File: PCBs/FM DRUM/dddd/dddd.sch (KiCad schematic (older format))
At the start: 44 parts, among them J1 Conn_02x12_Odd_Even, J2 Conn_01x03, J3 Conn_01x03, J4 Conn_01x03, J5 Conn_01x03, J6 Conn_01x03, J7 Conn_01x03, SW1 SW_DIP_x06, U1 LM555xM, U2 LM555xM, U3 MCP46x2, U4 LM555xM, U5 LM555xM, U6 MCP46x2, U7 MCP46x2, U8 TL072

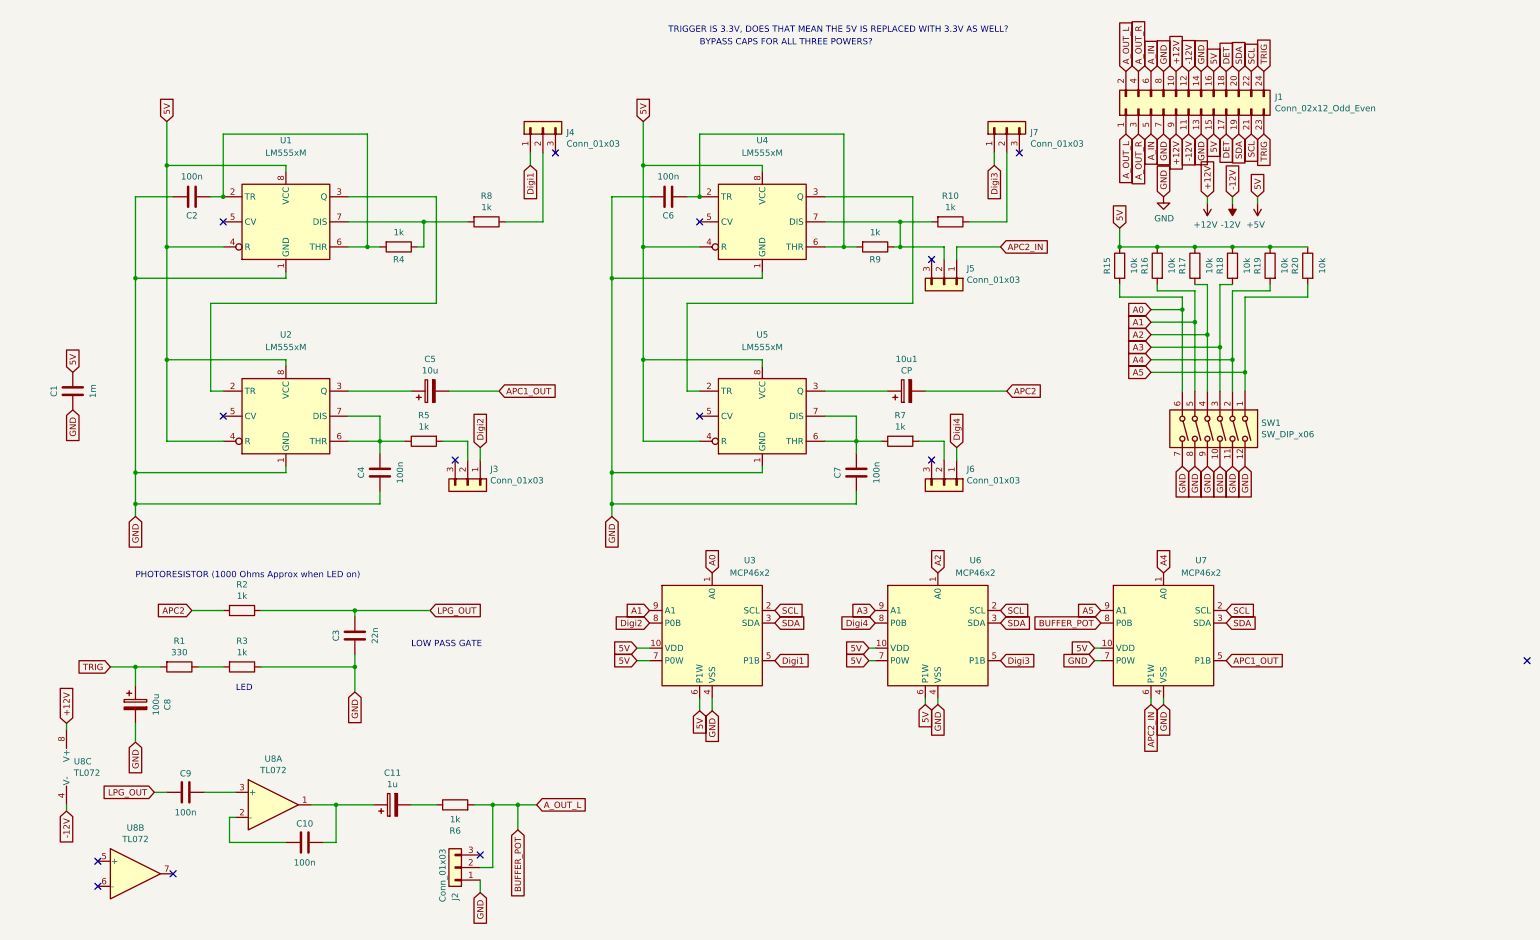
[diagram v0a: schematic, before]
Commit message: Add files via upload
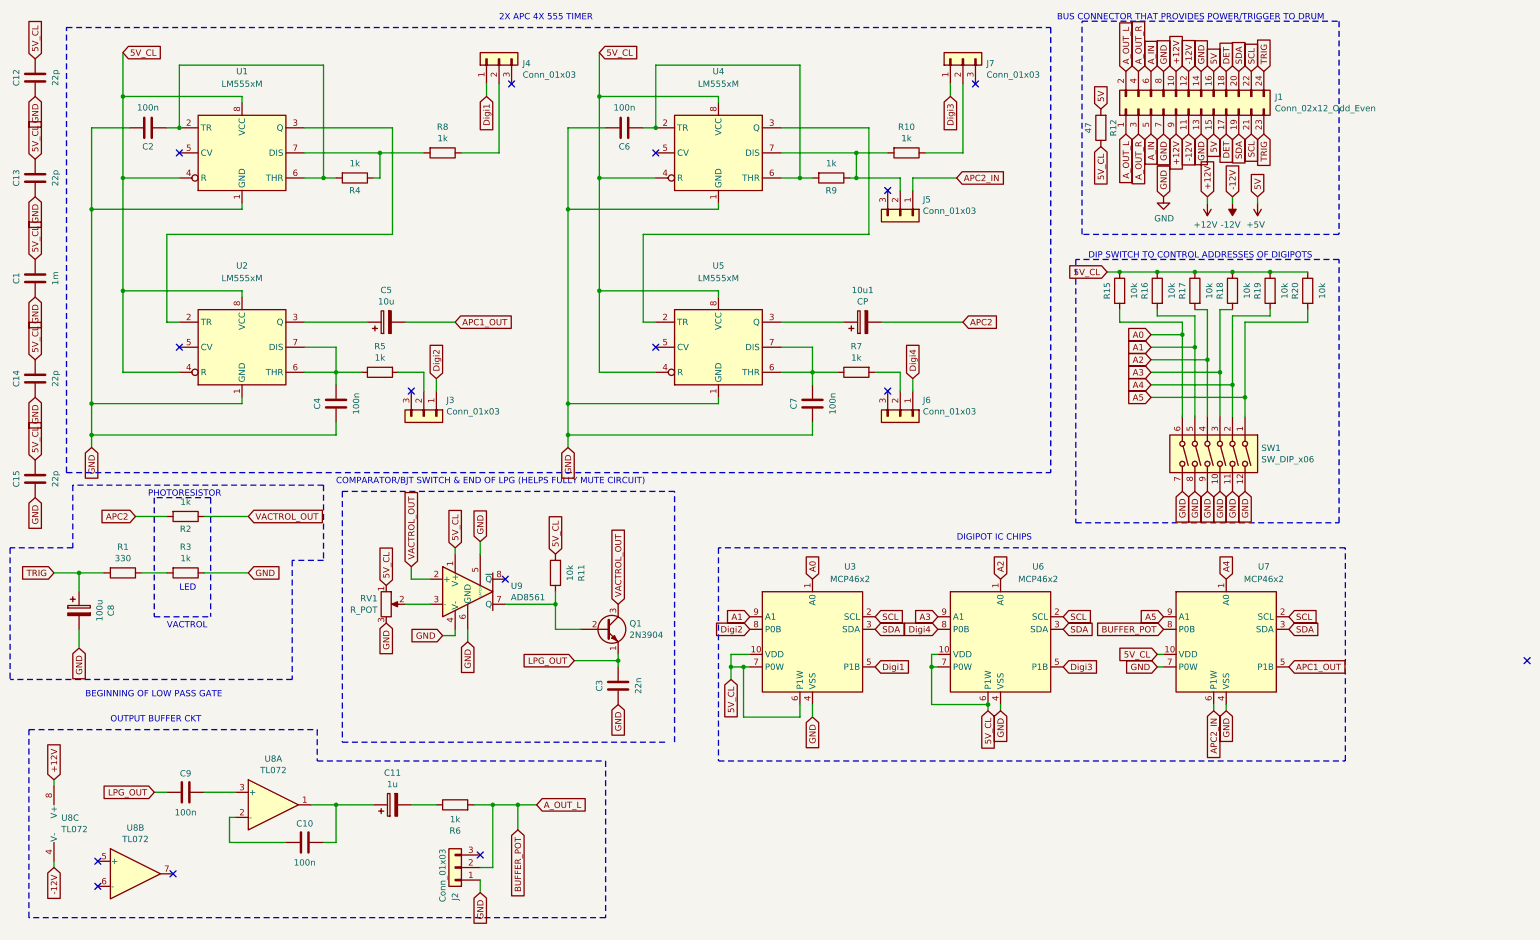
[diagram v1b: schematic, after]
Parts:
- added C12, C13, C14, C15: 22p, Resistor_THT:R_Axial_DIN0207_L6.3mm_D2.5mm_P5.08mm_Vertical, symbol Device:C
- added Q1: 2N3904, Connector_PinSocket_2.54mm:PinSocket_1x03_P2.54mm_Vertical, symbol Transistor_BJT:2N3904
- added R11: 10k, Resistor_THT:R_Axial_DIN0207_L6.3mm_D2.5mm_P10.16mm_Horizontal, symbol Device:R
- added R12: 47, Resistor_THT:R_Axial_DIN0207_L6.3mm_D2.5mm_P10.16mm_Horizontal, symbol Device:R
- added RV1: R_POT, Potentiometer_THT:Potentiometer_Piher_PT-6-V_Vertical, symbol Device:R_POT
- added U9: AD8561, Package_DIP:DIP-8_W7.62mm, symbol Comparator:AD8561
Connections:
- net +5V: now also R12.2; no longer C1.2, R15.1, R16.1, R17.1, R18.1, R19.1, R20.1, U1.4 (R), U1.8 (VCC), U2.4 (R), U2.8 (VCC), U3.10 (VDD), U3.6 (P1W), U3.7 (P0W), U4.4 (R), U4.8 (VCC), U5.4 (R), U5.8 (VCC), U6.10 (VDD), U6.6 (P1W), U6.7 (P0W), U7.10 (VDD)
- net GND: now also C12.1, C13.1, C14.1, C15.1, RV1.3, U9.4 (V-), U9.5 (LATCH), U9.6 (GND)
- net LPG_OUT: now also Q1.1 (E); no longer R2.1
- new net: RV1.2, U9.3 (-)
- new net: Q1.2 (B), R11.1, U9.7 (Q)
- new net 5V_CL: C1.2, C12.2, C13.2, C14.2, C15.2, R11.2, R12.1, R15.1, R16.1, R17.1, R18.1, R19.1, R20.1, RV1.1, U1.4 (R), U1.8 (VCC), U2.4 (R), U2.8 (VCC), U3.10 (VDD), U3.6 (P1W), U3.7 (P0W), U4.4 (R), U4.8 (VCC), U5.4 (R), U5.8 (VCC), U6.10 (VDD), U6.6 (P1W), U6.7 (P0W), U7.10 (VDD), U9.1 (V+)
- new net VACTROL_OUT: Q1.3 (C), R2.1, U9.2 (+)
- no-connect marks 14 -> 15
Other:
- note added: "2X APC 4X 555 TIMER"
- note added: "BEGINNING OF LOW PASS GATE"
- note added: "BUS CONNECTOR THAT PROVIDES POWER/TRIGGER TO DRUM"
- note added: "COMPARATOR/BJT SWITCH & END OF LPG (HELPS FULLY MUTE CIRCUIT)"
- note added: "DIGIPOT IC CHIPS"
- note added: "DIP SWITCH TO CONTROL ADDRESSES OF DIGIPOTS"
- note added: "OUTPUT BUFFER CKT"
- note added: "PHOTORESISTOR"
- note added: "VACTROL\n"
- note removed: "BYPASS CAPS FOR ALL THREE POWERS?\n"
- note removed: "LOW PASS GATE"
- note removed: "PHOTORESISTOR (1000 Ohms Approx when LED on)"
- note removed: "TRIGGER IS 3.3V, DOES THAT MEAN THE 5V IS REPLACED WITH 3.3V AS WELL?"
- moved on the sheet: 10u1, C1, C2, C3, C4, C5, C6, C7, C8, J3, J4, J5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
